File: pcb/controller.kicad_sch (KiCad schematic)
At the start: 65 parts, among them J16 uC_NRST, J17 3V3_uC, J18 SWO, J4 DEBUG, J5 UART, U2 SN65HVD234, U3 STM32F103RETx, Y1 8MHz

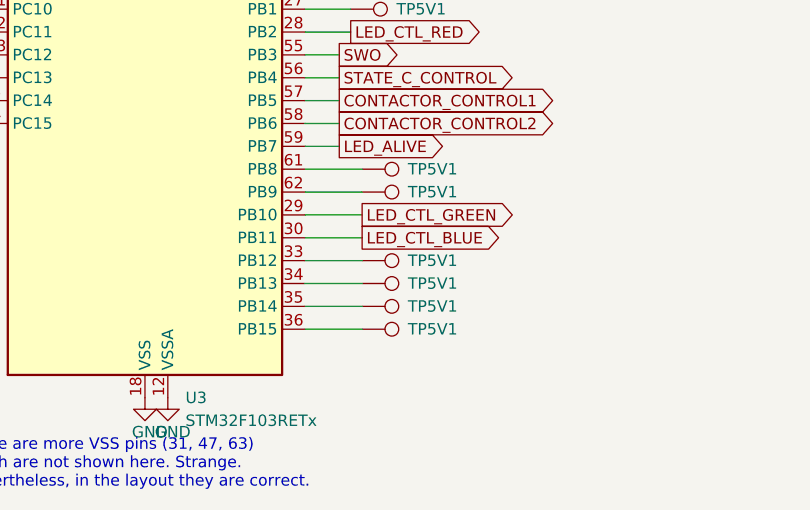
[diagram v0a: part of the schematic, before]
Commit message: wired the drv8874. Added spare holes. Flash connector larger holes
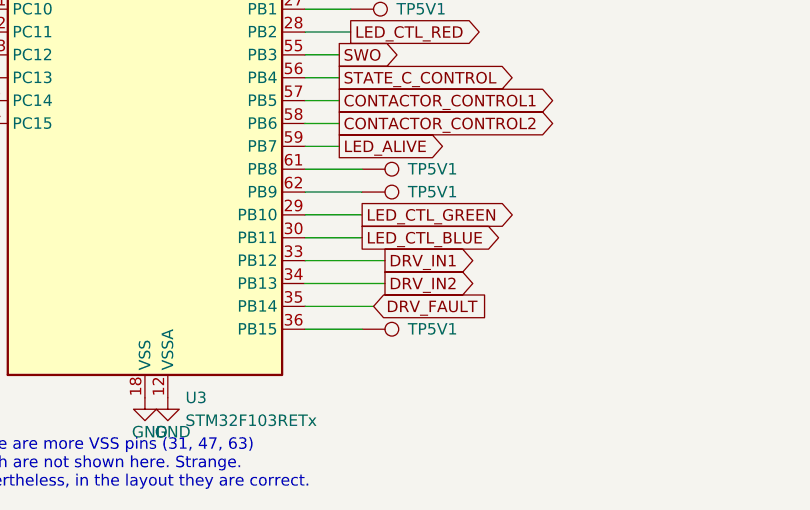
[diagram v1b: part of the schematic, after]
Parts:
- removed TP5V1 (x3): ~, TestPoint:TestPoint_THTPad_D1.0mm_Drill0.5mm, symbol Connector:TestPoint
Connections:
- net DRV_IN2: now reaches U3.34 (PB13)
- net DRV_IN1: now reaches U3.33 (PB12)
- net DRV_FAULT: now reaches U3.35 (PB14)
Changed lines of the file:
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@@
     (stroke (width 0) (type default))
   )
-  (wire (pts (xy 171.45 143.51) (xy 177.8 143.51))
+  (wire (pts (xy 171.45 143.51) (xy 179.07 143.51))
     (stroke (width 0) (type default))
   )
@@
     (stroke (width 0) (type default))
   )
-  (wire (pts (xy 171.45 140.97) (xy 177.8 140.97))
+  (wire (pts (xy 171.45 140.97) (xy 180.34 140.97))
     (stroke (width 0) (type default))
   )
@@
     (stroke (width 0) (type default))
   )
-  (wire (pts (xy 171.45 138.43) (xy 177.8 138.43))
+  (wire (pts (xy 171.45 138.43) (xy 180.34 138.43))
     (stroke (width 0) (type default))
   )
@@
     )
   )
+  (global_label "DRV_IN1" (shape output) (at 180.34 138.43 0) (fields_autoplaced)
+    (effects (font (size 1.27 1.27)) (justify left))
+    (property "Intersheetrefs" "${INTERSHEET_REFS}" (at 190.9868 138.43 0)
+      (effects (font (size 1.27 1.27)) (justify left) hide)
+    )
+  )
   (global_label "SERIAL_IO_2_CS" (shape input) (at 240.03 40.64 0) (fields_autoplaced)
     (effects (font (size 1.27 1.27)) (justify left))
@@
     )
   )
+  (global_label "DRV_FAULT" (shape input) (at 179.07 143.51 0) (fields_autoplaced)
+    (effects (font (size 1.27 1.27)) (justify left))
+    (property "Intersheetrefs" "${INTERSHEET_REFS}" (at 192.0754 143.51 0)
+      (effects (font (size 1.27 1.27)) (justify left) hide)
+    )
+  )
   (global_label "ADC123_IN10" (shape input) (at 130.81 85.09 180) (fields_autoplaced)
     (effects (font (size 1.27 1.27)) (justify right))
@@
     )
   )
+  (global_label "DRV_IN2" (shape output) (at 180.34 140.97 0) (fields_autoplaced)
+    (effects (font (size 1.27 1.27)) (justify left))
+    (property "Intersheetrefs" "${INTERSHEET_REFS}" (at 190.9868 140.97 0)
+      (effects (font (size 1.27 1.27)) (justify left) hide)
+    )
+  )
   (global_label "CONTACTOR_CONTROL1" (shape input) (at 44.45 123.19 180) (fields_autoplaced)
     (effects (font (size 1.27 1.27)) (justify right))
@@
     )
   )
-  (symbol (lib_id "Connector:TestPoint") (at 177.8 140.97 270) (unit 1)
-    (in_bom yes) (on_board yes) (dnp no)
-    (property "Reference" "TP5V1" (at 182.88 140.97 90)
-      (effects (font (size 1.27 1.27)) (justify left))
-    )
-    (property "Value" "~" (at 182.88 139.7 0)
-      (effects (font (size 1.27 1.27)) (justify left))
-    )
-    (property "Footprint" "TestPoint:TestPoint_THTPad_D1.0mm_Drill0.5mm" (at 177.8 146.05 0)
-      (effects (font (size 1.27 1.27)) hide)
-    )
-    (property "Datasheet" "~" (at 177.8 146.05 0)
-      (effects (font (size 1.27 1.27)) hide)
-    )
-    (pin "1")
-    (instances
-      (project "qca7000"
-        (path "/e63e39d7-6ac0-4ffd-8aa3-1841a4541b55"
-          (reference "TP5V1") (unit 1)
-        )
-        (path "/e63e39d7-6ac0-4ffd-8aa3-1841a4541b55/81db238c-e53f-4d52-98ea-36a1df697651"
-          (reference "TP5V1") (unit 1)
-        )
-        (path "/e63e39d7-6ac0-4ffd-8aa3-1841a4541b55/5666e7cf-6b6c-4583-8335-aa3be69ccd45"
-          (reference "TP36") (unit 1)
-        )
-      )
-    )
-  )
   (symbol (lib_id "Connector:TestPoint") (at 133.35 102.87 90) (unit 1)
     (in_bom yes) (on_board yes) (dnp no)
@@
     )
   )
-  (symbol (lib_id "Connector:TestPoint") (at 177.8 138.43 270) (unit 1)
-    (in_bom yes) (on_board yes) (dnp no)
-    (property "Reference" "TP5V1" (at 182.88 138.43 90)
-      (effects (font (size 1.27 1.27)) (justify left))
-    )
-    (property "Value" "~" (at 182.88 137.16 0)
-      (effects (font (size 1.27 1.27)) (justify left))
-    )
-    (property "Footprint" "TestPoint:TestPoint_THTPad_D1.0mm_Drill0.5mm" (at 177.8 143.51 0)
-      (effects (font (size 1.27 1.27)) hide)
-    )
-    (property "Datasheet" "~" (at 177.8 143.51 0)
-      (effects (font (size 1.27 1.27)) hide)
-    )
-    (pin "1")
-    (instances
-      (project "qca7000"
-        (path "/e63e39d7-6ac0-4ffd-8aa3-1841a4541b55"
-          (reference "TP5V1") (unit 1)
-        )
-        (path "/e63e39d7-6ac0-4ffd-8aa3-1841a4541b55/81db238c-e53f-4d52-98ea-36a1df697651"
-          (reference "TP5V1") (unit 1)
-        )
-        (path "/e63e39d7-6ac0-4ffd-8aa3-1841a4541b55/5666e7cf-6b6c-4583-8335-aa3be69ccd45"
-          (reference "TP34") (unit 1)
-        )
-      )
-    )
-  )
   (symbol (lib_id "Connector:Conn_01x03_Pin") (at 256.54 154.94 180) (unit 1)
     (in_bom yes) (on_board yes) (dnp no) (fields_autoplaced)
@@
         )
       )
-    )
-  )
-  (symbol (lib_id "Connector:TestPoint") (at 177.8 143.51 270) (unit 1)
-    (in_bom yes) (on_board yes) (dnp no)
-    (property "Reference" "TP5V1" (at 182.88 143.51 90)
-      (effects (font (size 1.27 1.27)) (justify left))
-    )
-    (property "Value" "~" (at 182.88 142.24 0)
-      (effects (font (size 1.27 1.27)) (justify left))
-    )
-    (property "Footprint" "TestPoint:TestPoint_THTPad_D1.0mm_Drill0.5mm" (at 177.8 148.59 0)
-      (effects (font (size 1.27 1.27)) hide)
-    )
-    (property "Datasheet" "~" (at 177.8 148.59 0)
-      (effects (font (size 1.27 1.27)) hide)
-    )
-    (pin "1")
-    (instances
-      (project "qca7000"
-        (path "/e63e39d7-6ac0-4ffd-8aa3-1841a4541b55"
-          (reference "TP5V1") (unit 1)
-        )
-        (path "/e63e39d7-6ac0-4ffd-8aa3-1841a4541b55/81db238c-e53f-4d52-98ea-36a1df697651"
-          (reference "TP5V1") (unit 1)
-        )
-        (path "/e63e39d7-6ac0-4ffd-8aa3-1841a4541b55/5666e7cf-6b6c-4583-8335-aa3be69ccd45"
-          (reference "TP37") (unit 1)
-        )
-      )
